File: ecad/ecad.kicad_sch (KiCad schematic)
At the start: 44 parts, among them J1 JTAG, J2 USB_C, J3 Display, Q1 SS8050, SW10 RotaryEncoder_Switch, SW11 RotaryEncoder_Switch, SW15 RESET, SW24 Kailh choc v2, SW25 Kailh choc v2, U1 AP2112K-3.3, U2 RP2040, U5 W25Q128JVP, Y1 12MHz

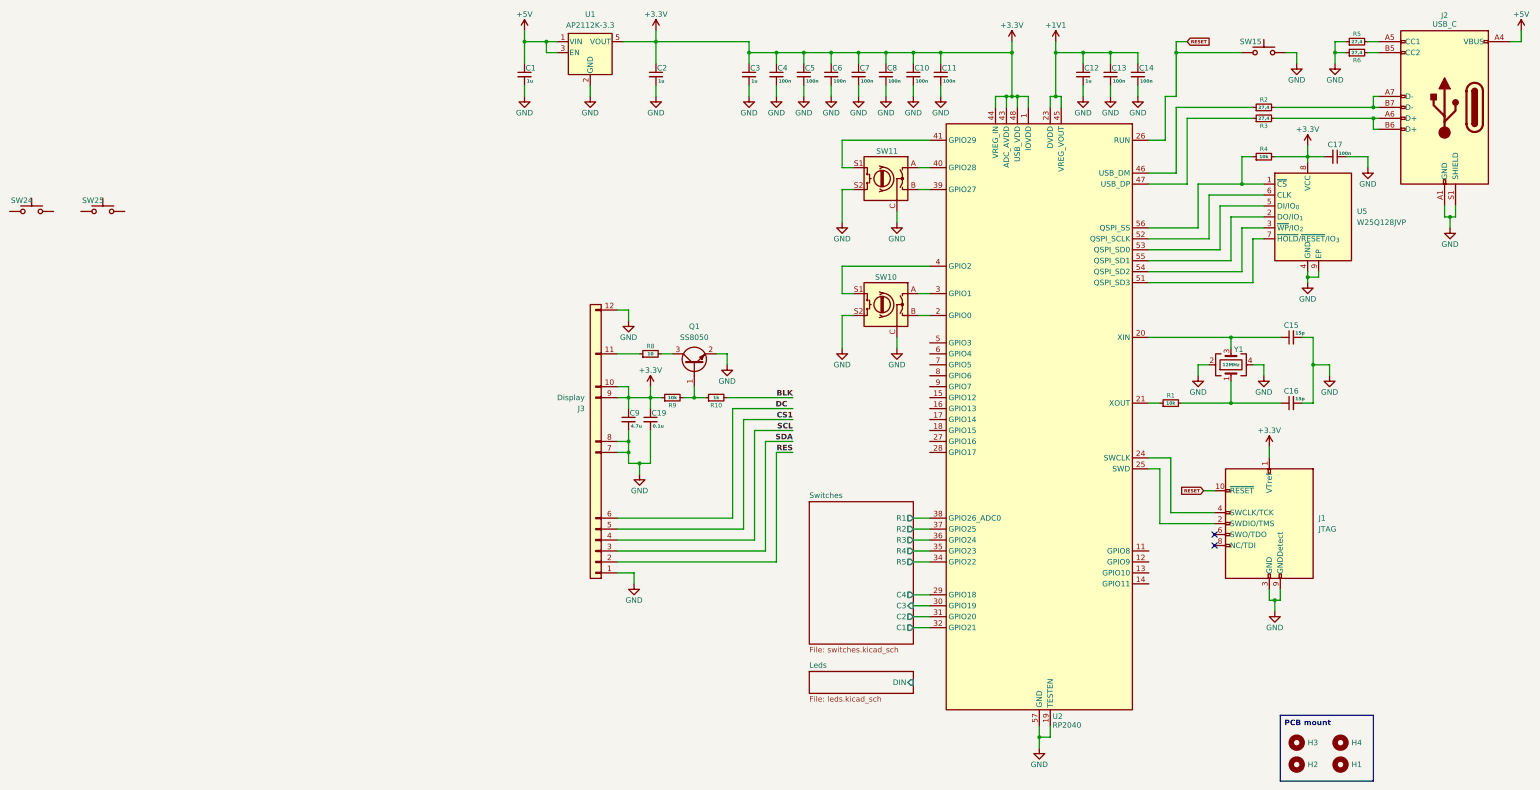
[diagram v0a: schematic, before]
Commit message: feat(ecad): general routing
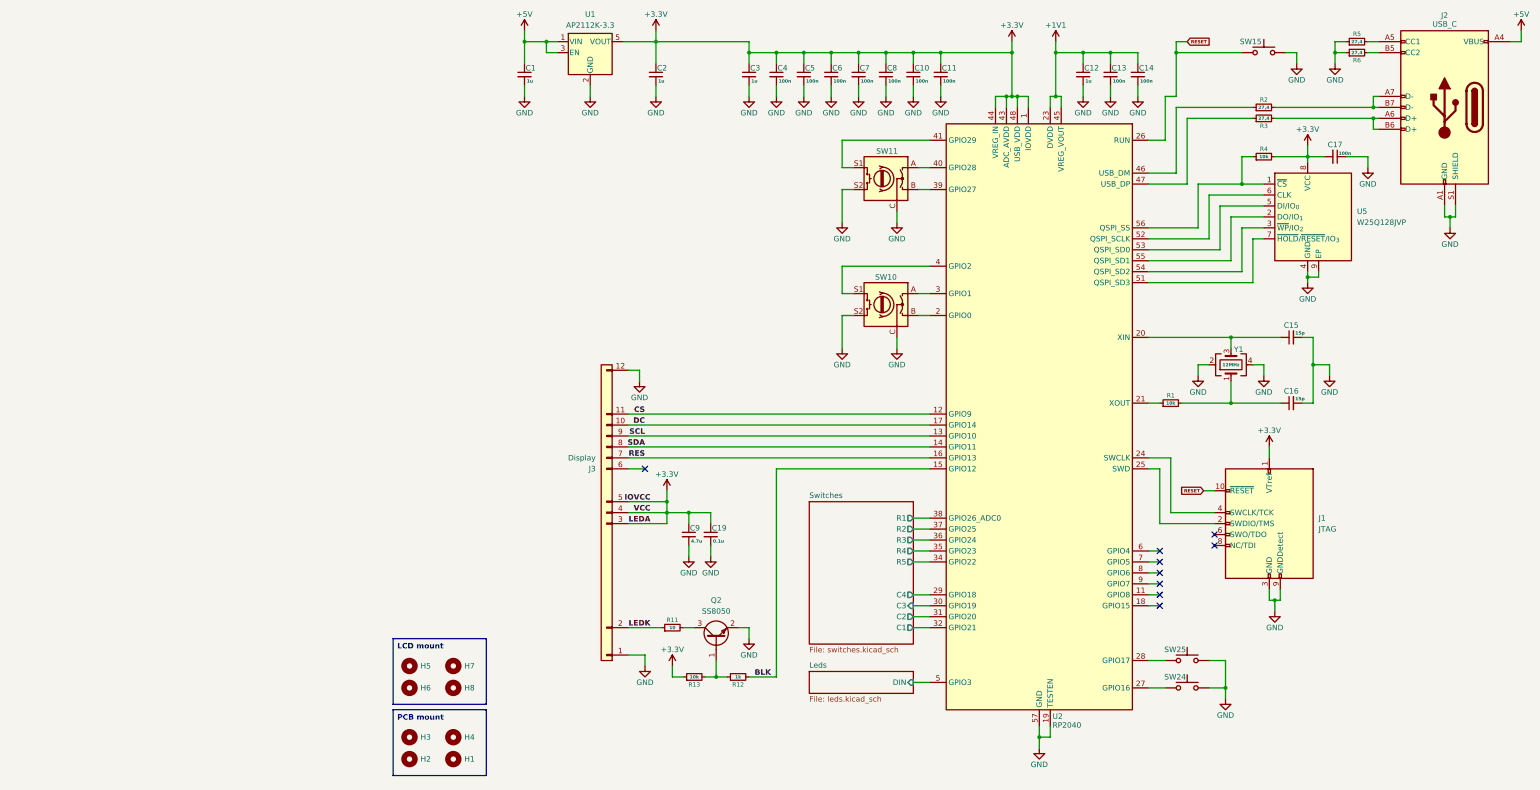
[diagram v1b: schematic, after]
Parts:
- removed Q1: SS8050, Package_TO_SOT_SMD:SOT-23, symbol Transistor_BJT:SS8050
- removed R10: 1k, Resistor_SMD:R_0402_1005Metric, symbol Device:R_Small
- removed R8: 10, Resistor_SMD:R_0402_1005Metric, symbol Device:R_Small
- removed R9: 10k, Resistor_SMD:R_0402_1005Metric, symbol Device:R_Small
- added H5, H6, H7, H8: MountingHole, MountingHole:MountingHole_2.2mm_M2_DIN965, symbol Mechanical:MountingHole
- added Q2: SS8050, Package_TO_SOT_SMD:SOT-23, symbol Transistor_BJT:SS8050
- added R11: 10, Resistor_SMD:R_0402_1005Metric, symbol Device:R_Small
- added R12: 1k, Resistor_SMD:R_0402_1005Metric, symbol Device:R_Small
- added R13: 10k, Resistor_SMD:R_0402_1005Metric, symbol Device:R_Small
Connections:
- net CS1 is gone; now on net +3.3V: J3.5 (Pin_5)
- net +3.3V: now also J3.3 (Pin_3), J3.4 (Pin_4), R13.1; no longer J3.10 (Pin_10), J3.9 (Pin_9)
- net BLK: now also U2.15 (GPIO12), R12.2
- net DC: now also J3.10 (Pin_10), U2.17 (GPIO14); no longer J3.6 (Pin_6)
- net GND: now also SW24.2, SW25.2, Q2.2 (E); no longer J3.7 (Pin_7), J3.8 (Pin_8)
- net Leds/DIN: now also U2.5 (GPIO3)
- net RES: now also J3.7 (Pin_7), U2.16 (GPIO13); no longer J3.2 (Pin_2)
- net SCL: now also J3.9 (Pin_9), U2.13 (GPIO10); no longer J3.4 (Pin_4)
- net SDA: now also J3.8 (Pin_8), U2.14 (GPIO11); no longer J3.3 (Pin_3)
- net CS: now reaches J3.11 (Pin_11)
- net CS: now also U2.12 (GPIO9)
- net at SW24.1: now also U2.27 (GPIO16)
- net at SW25.1: now also U2.28 (GPIO17)
- new net: Q2.1 (B), R12.1, R13.2
- new net: Q2.3 (C), R11.2
- new net LEDK: J3.2 (Pin_2), R11.1
- no-connect marks 2 -> 9
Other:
- moved on the sheet: C19, C9, H1, H2, H3, H4, J3, SW24, SW25
